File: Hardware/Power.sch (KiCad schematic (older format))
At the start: 20 parts, among them U1 TPS63031DSKR, U2 TPS63002

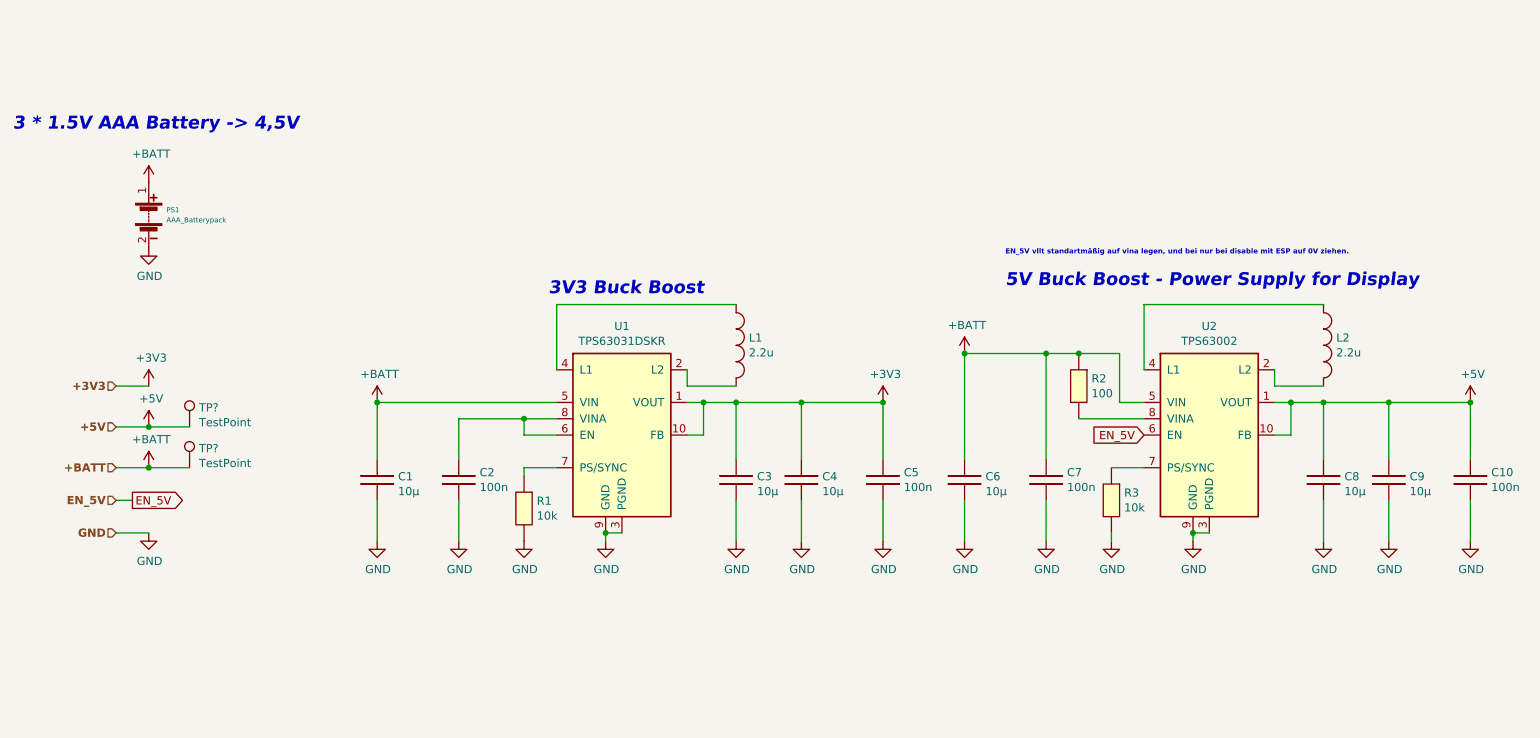
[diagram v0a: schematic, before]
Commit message: Martin ist unförmig
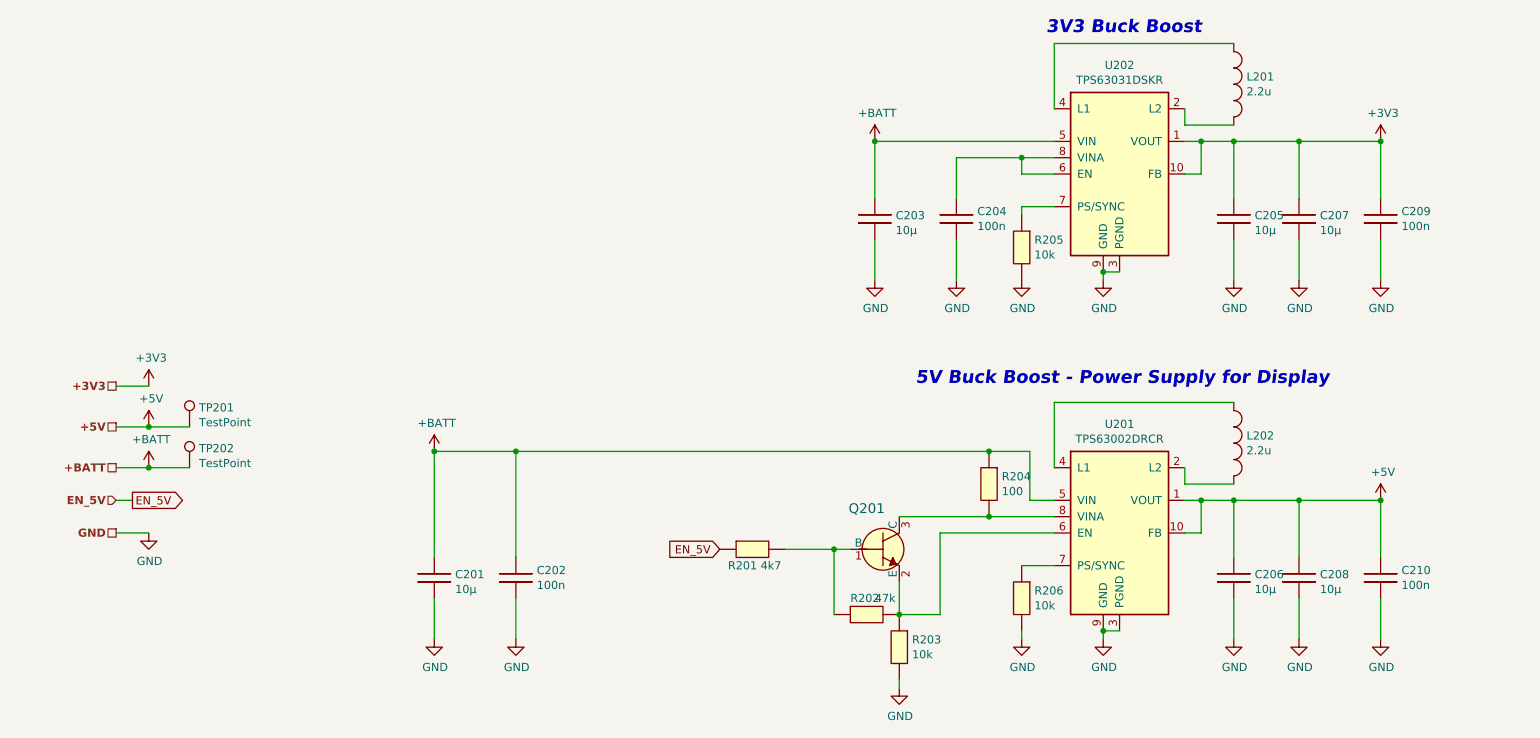
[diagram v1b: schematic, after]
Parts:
- removed PS1: AAA_Batterypack, symbol E-Ink:AAA_Batterypack
- added Q201: BC847B_215-dk_Transistors-Bipolar-BJT-Single, digikey-footprints:SOT-23-3, symbol E-Ink-rescue:BC847B_215-dk_Transistors-Bipolar-BJT-Single
- added R201: 4k7, Resistor_SMD:R_0805_2012Metric_Pad1.15x1.40mm_HandSolder, symbol E-Ink:4k7
- added R202: 47k, Resistor_SMD:R_0805_2012Metric_Pad1.15x1.40mm_HandSolder, symbol E-Ink:47k
- added R203: 10k, Resistor_SMD:R_0805_2012Metric_Pad1.15x1.40mm_HandSolder, symbol E-Ink:10k
- L201: renamed from L1; footprint (none) -> E-Ink:L_Taiyo-Yuden_MD-3030
- L202: renamed from L2; footprint (none) -> E-Ink:L_Taiyo-Yuden_MD-3030
- TP201, TP202: renamed from TP?; footprint (none) -> digikey-footprints:Test_Point_D1.02mm; Digi-Key_PN (none) -> 36-5001-ND
- U201: renamed from U2; value TPS63002 -> TPS63002DRCR
- U202: renamed from U1; footprint Package_SON:Texas_S-PWSON-N10 -> E-Ink:WSON-8-1EP_3x3mm_P0.5mm_EP1.6x2.0mm
- renumbered C6 to C201, C7 to C202, C1 to C203, C2 to C204, C3 to C205, C8 to C206, C4 to C207, C9 to C208, C5 to C209, C10 to C210, R2 to R204, R1 to R205, R3 to R206
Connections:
- net EN_5V: now also R201.1; no longer U201.6 (EN)
- net GND: now also R203.2
- net at R204.2, U201.8 (VINA): now also Q201.3 (C)
- new net: Q201.2 (E), R202.2, R203.1, U201.6 (EN)
- new net: Q201.1 (B), R201.2, R202.1
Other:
- note removed: "3 * 1.5V AAA Battery -> 4,5V"
- note removed: "EN_5V vllt standartmäßig auf vina legen, und bei nur bei disable mit ESP auf 0V ziehen."
- moved on the sheet: C201, C202, C203, C204, C205, C206, C207, C208, C209, C210, L201, L202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

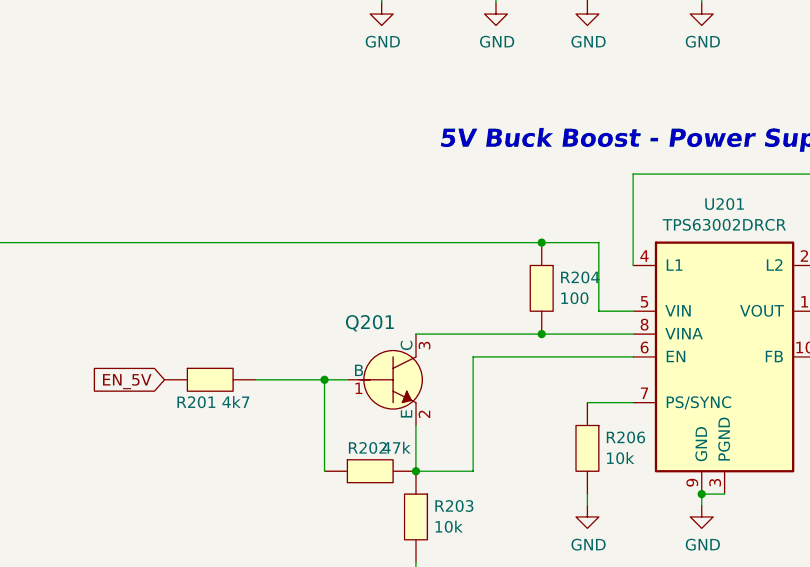
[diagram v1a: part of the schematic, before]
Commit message: Ich hoffe wir koennen jetzt den Master mergen!
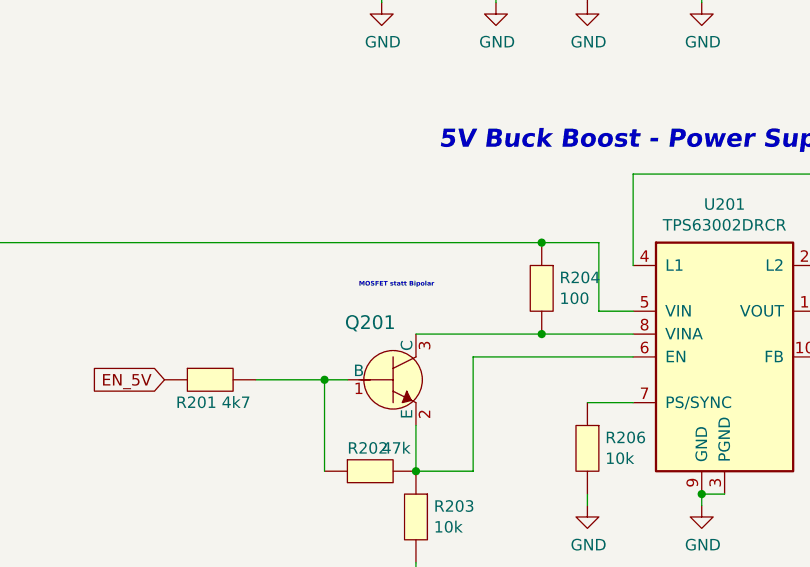
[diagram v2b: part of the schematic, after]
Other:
- note added: "MOSFET statt Bipolar\n"
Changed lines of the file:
@@
 Wire Wire Line
 	6650 4250 7350 4250
+Text Notes 6150 3950 0    20   ~ 4
+MOSFET statt Bipolar\n
 $EndSCHEMATC
